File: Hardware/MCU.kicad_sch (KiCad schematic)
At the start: 31 parts, among them J3 Conn_01x04_Pin, SW1 SW_Push, SW2 SW_SPDT, U1 STM32F405RGTx, Y1 25Mhz

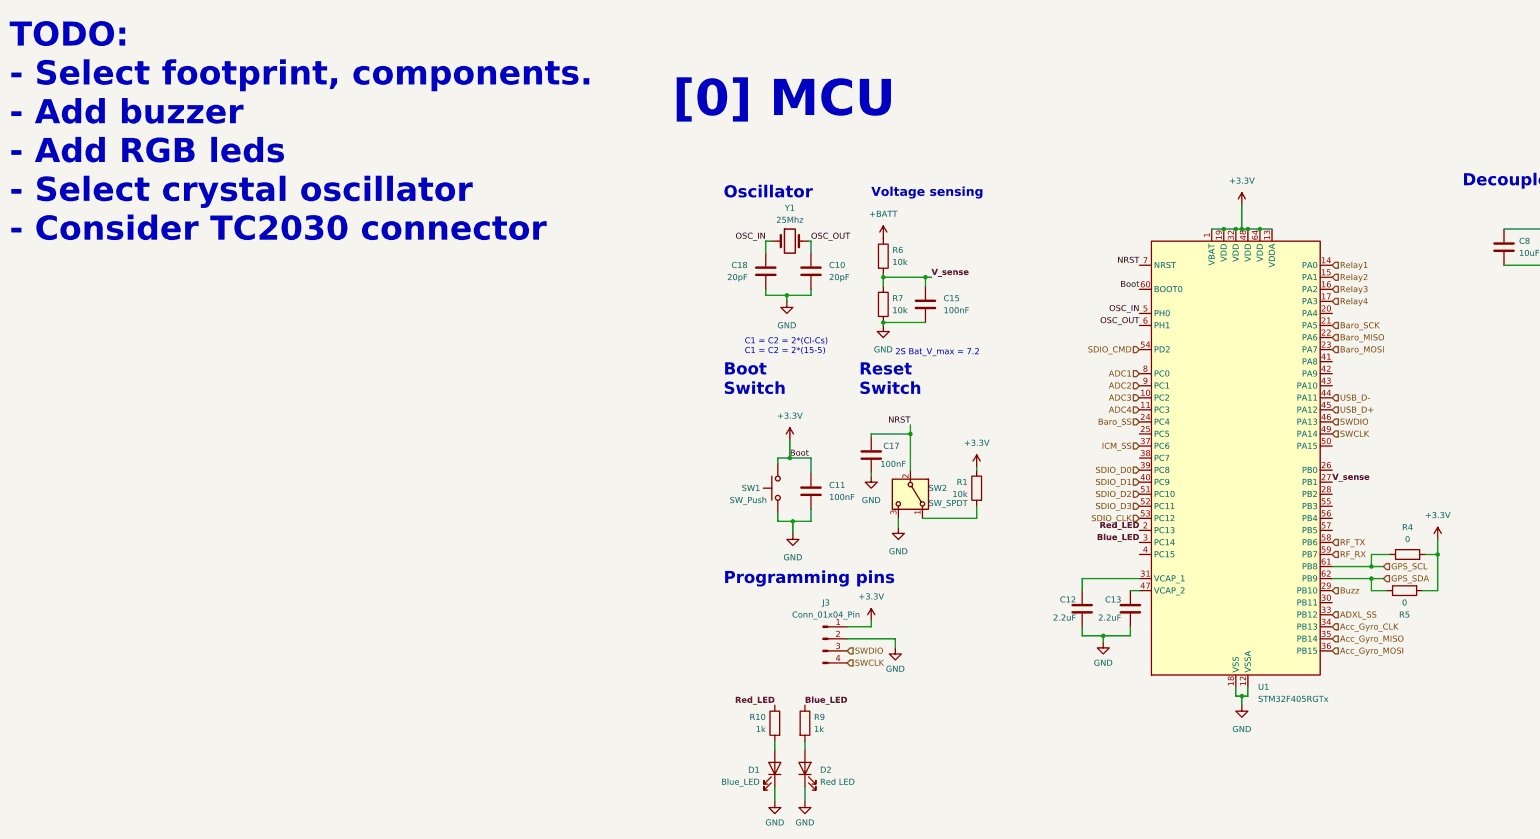
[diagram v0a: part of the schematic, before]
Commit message: Added a simulations file, added App Notes file, Finalized SD-card design type shit
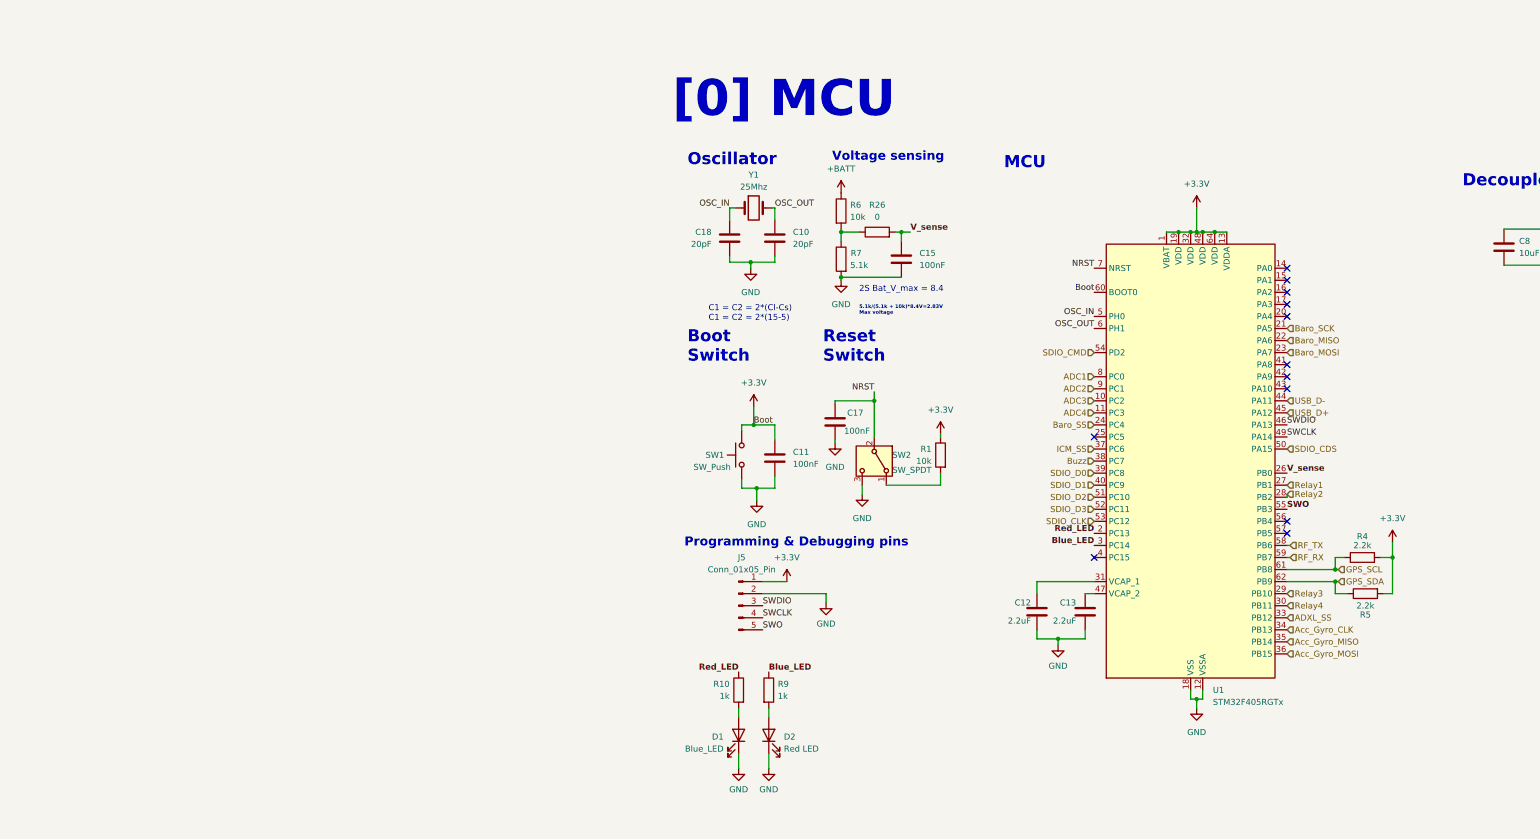
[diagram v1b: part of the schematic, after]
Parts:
- removed J3: Conn_01x04_Pin, Connector_PinHeader_2.54mm:PinHeader_1x04_P2.54mm_Vertical, symbol Connector:Conn_01x04_Pin
- added J5: Conn_01x05_Pin, symbol Connector:Conn_01x05_Pin
- added R26: 0, Resistor_SMD:R_0402_1005Metric, symbol Device:R
- R1, R6: Distributer Link https://www.ozdisan.com/p/smt-smd-ve-cip-direncler-194/roya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 -> https://www.ozdisan.com/p/smt-smd-ve-cip-direncler-194/pana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; Part Number CQ03SAJ0103T5E -> ERJ3EKF1002V
- R4, R5: value 0 -> 2.2k
- R7: value 10k -> 5.1k; footprint Resistor_SMD:R_0603_1608Metric -> Resistor_SMD:R_0402_1005Metric; Distributer Link https://www.ozdisan.com/p/smt-smd-ve-cip-direncler-194/roya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 -> https://www.ozdisan.com/p/smt-smd-ve-cip-direncler-194/pana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; Part Number CQ03SAJ0103T5E -> ERJ2RKF5101X
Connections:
- net +3.3V: now also J5.1 (Pin_1)
- net Buzz: now also U1.38 (PC7); no longer U1.29 (PB10)
- net GND: now also J5.2 (Pin_2)
- net Relay1: now also U1.27 (PB1); no longer U1.14 (PA0)
- net Relay2: now also U1.28 (PB2); no longer U1.15 (PA1)
- net Relay3: now also U1.29 (PB10); no longer U1.16 (PA2)
- net Relay4: now also U1.30 (PB11); no longer U1.17 (PA3)
- net SWCLK: now also J5.4 (Pin_4)
- net SWDIO: now also J5.3 (Pin_3)
- net V_sense: now also U1.26 (PB0), R26.2; no longer R6.2, R7.1, U1.27 (PB1)
- net SDIO_CDS: now reaches U1.50 (PA15)
- net SWO: now reaches U1.55 (PB3)
- net SWO: now also J5.5 (Pin_5)
- new net: R26.1, R6.2, R7.1
- no-connect marks 0 -> 12
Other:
- note added: "2S Bat_V_max = 8.4"
- note added: "5.1k/(5.1k + 10k)*8.4V=2.83V Max voltage"
- note added: "MCU"
- note added: "Programming & Debugging pins"
- note removed: "2S Bat_V_max = 7.2"
- note removed: "Programming pins"
- note removed: "TODO: - Select footprint, components. - Add buzzer - Add RGB leds - Select crystal oscillator - Consider TC2030 connector"
- moved on the sheet: C10, C11, C12, C13, C15, C17, C18, D1, D2, R1, R10, R4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

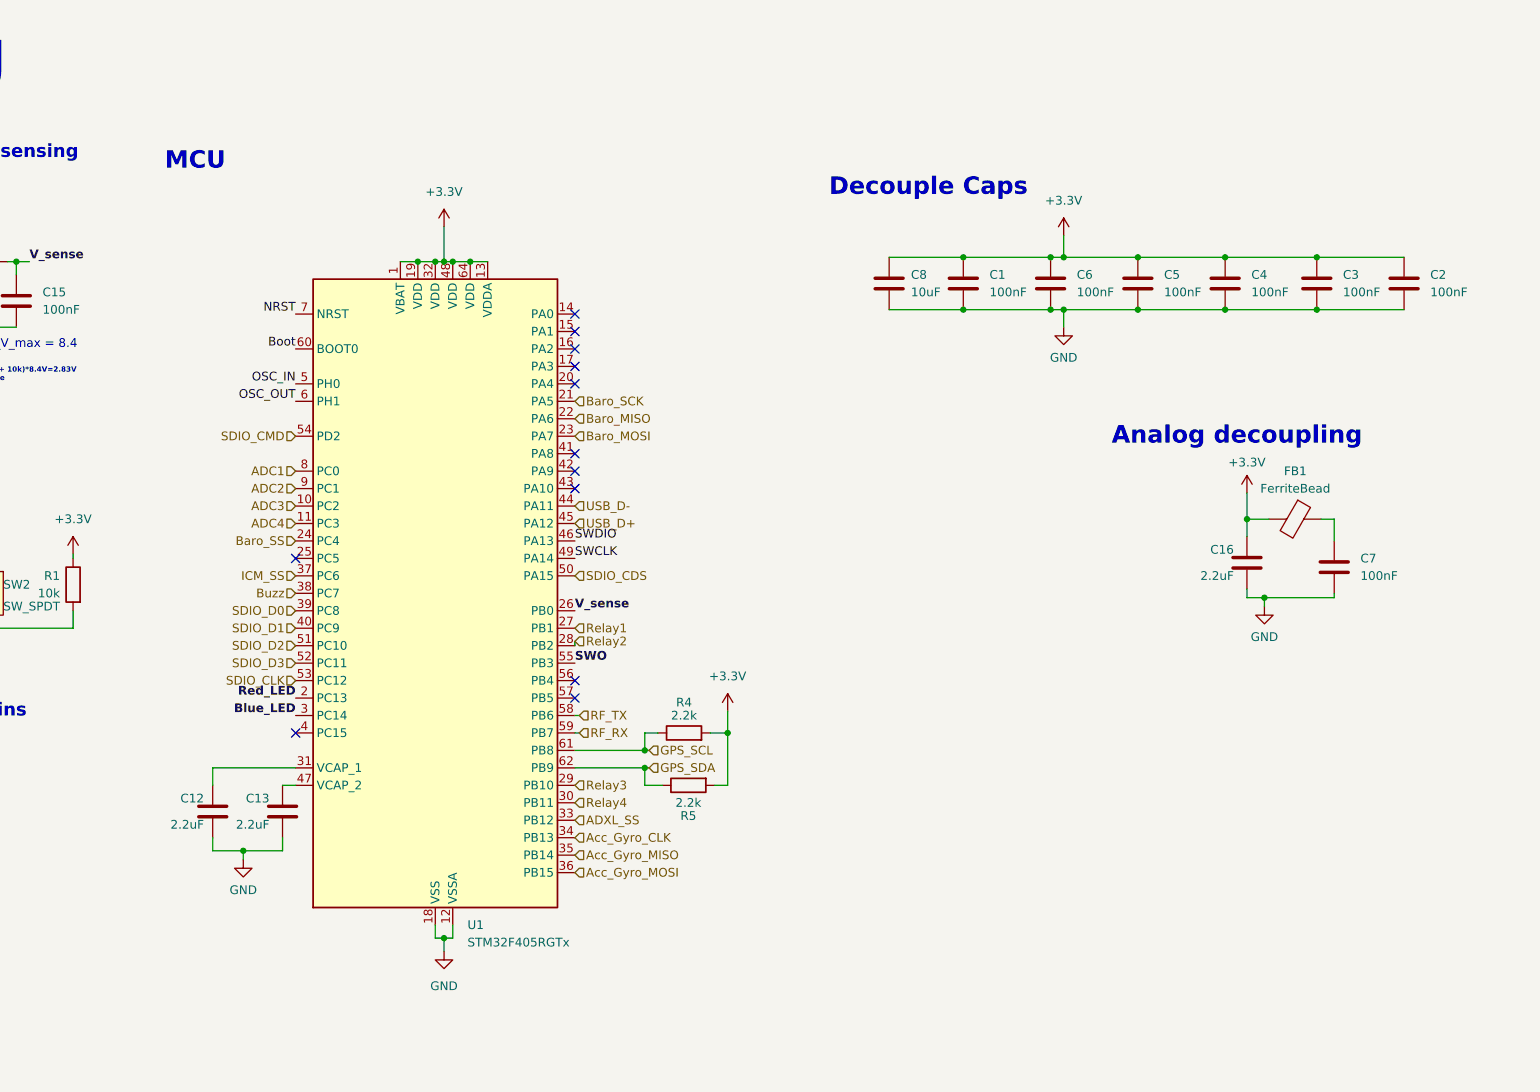
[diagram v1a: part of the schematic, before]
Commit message: +1000 Aura
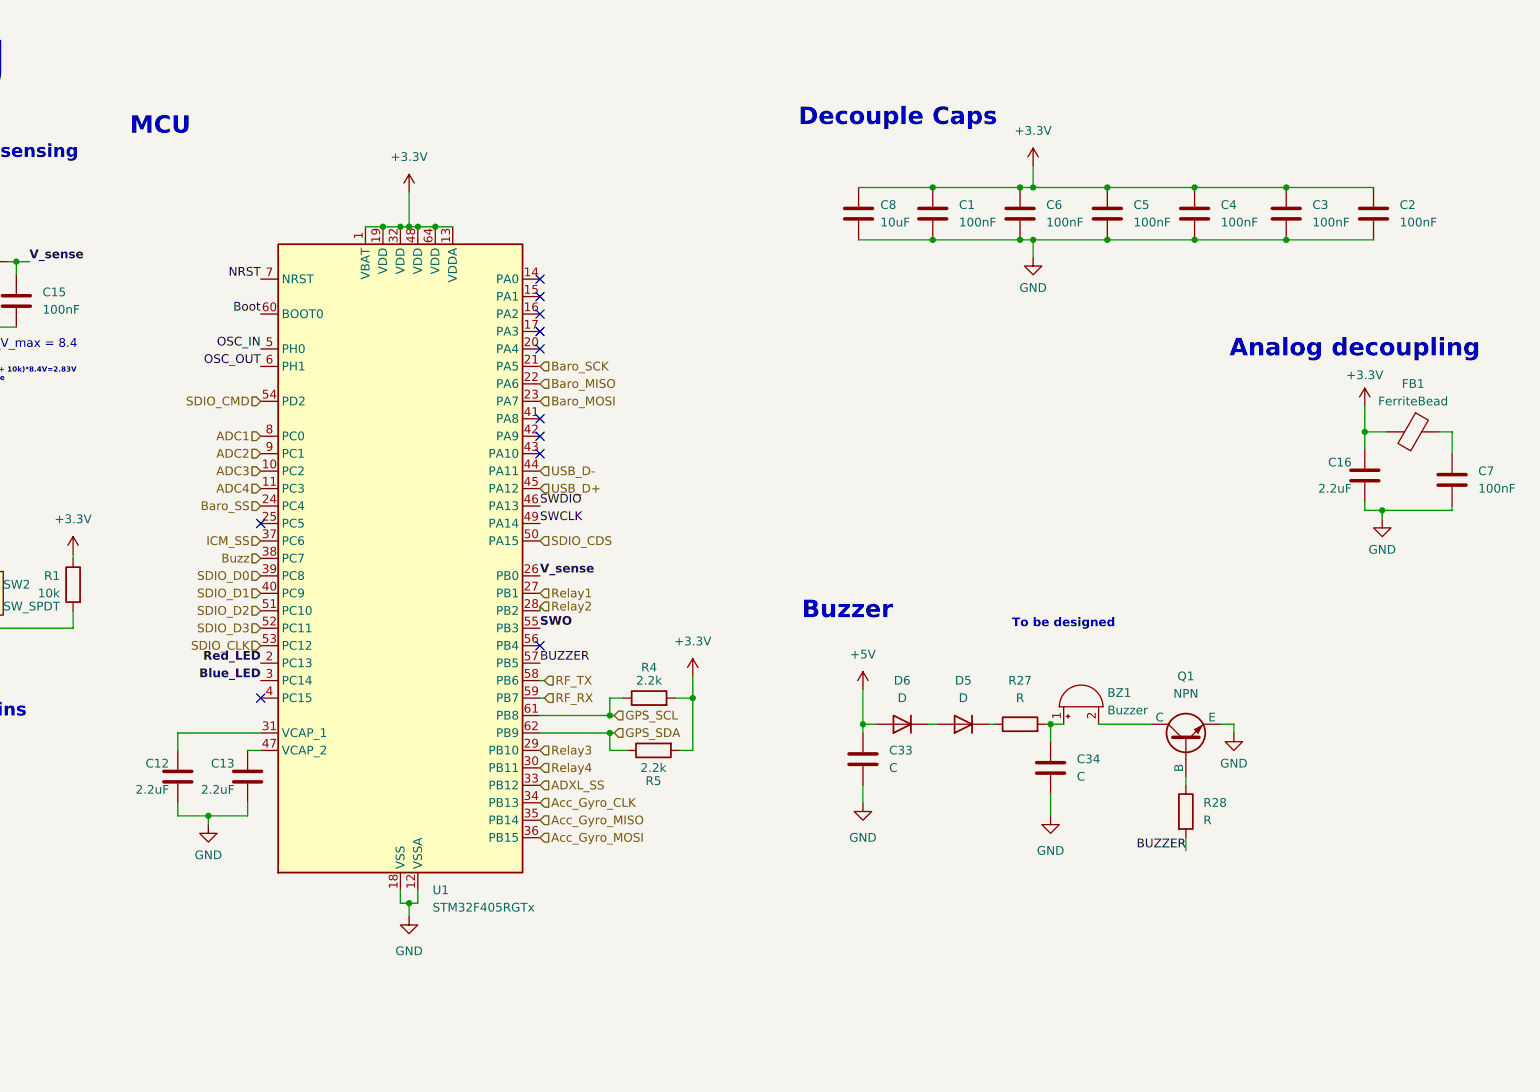
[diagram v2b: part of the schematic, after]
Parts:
- added BZ1: Buzzer, symbol Device:Buzzer
- added C33, C34: C, symbol Device:C
- added D5, D6: D, symbol Device:D
- added Q1: NPN, symbol Simulation_SPICE:NPN
- added R27, R28: R, symbol Device:R
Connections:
- net GND: now also C33.2, C34.2, Q1.3 (E)
- net BUZZER: now reaches U1.57 (PB5)
- net BUZZER: now also R28.2
- new net: BZ1.2 (-), Q1.1 (C)
- new net: Q1.2 (B), R28.1
- new net: D5.1 (K), R27.1
- new net: BZ1.1 (+), C34.1, R27.2
- new net: D5.2 (A), D6.1 (K)
- new net +5V: C33.1, D6.2 (A)
- no-connect marks 12 -> 11
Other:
- note added: "Buzzer"
- note added: "To be designed"
- moved on the sheet: C1, C12, C13, C16, C2, C3, C4, C5, C6, C7, C8, FB1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
